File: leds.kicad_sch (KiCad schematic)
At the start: 5 parts, among them J28 JST PH 3, U1 74AHCT1G32SE-7

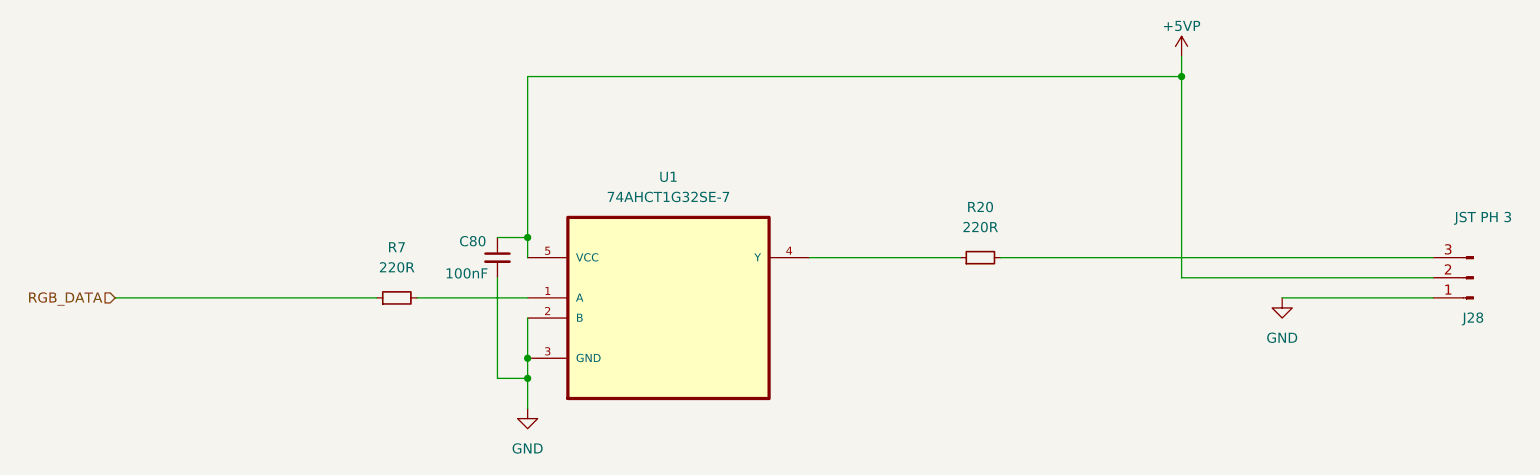
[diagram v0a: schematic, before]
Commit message: fixed warnings.
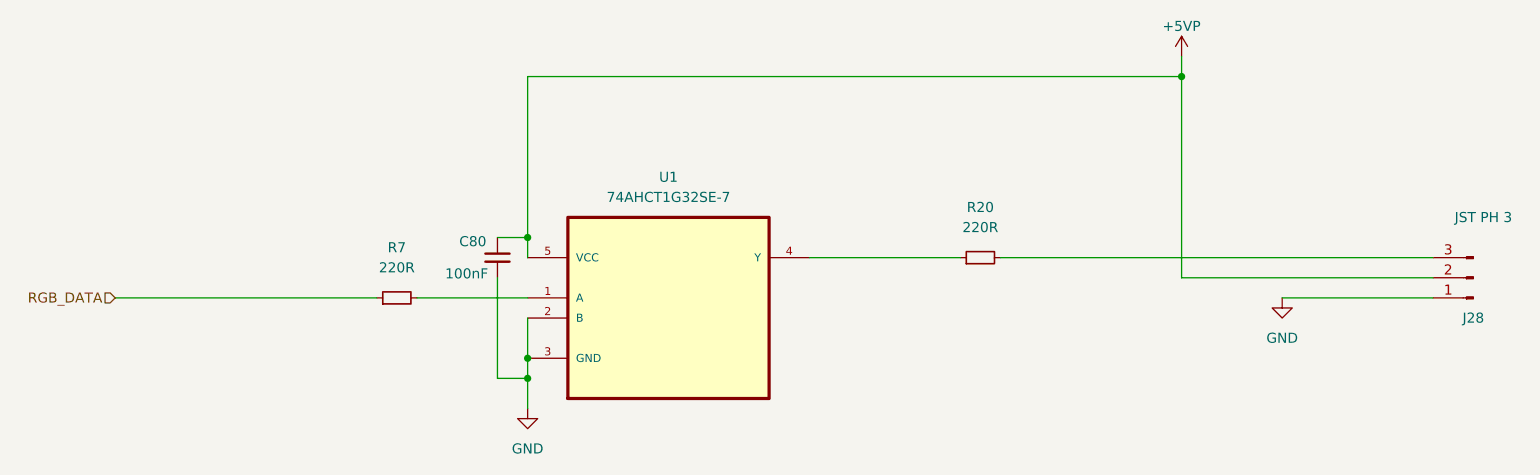
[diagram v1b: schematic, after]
